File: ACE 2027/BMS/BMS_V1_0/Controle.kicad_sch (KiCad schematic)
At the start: 9 parts, among them J205 RJ45, J206 RJ45

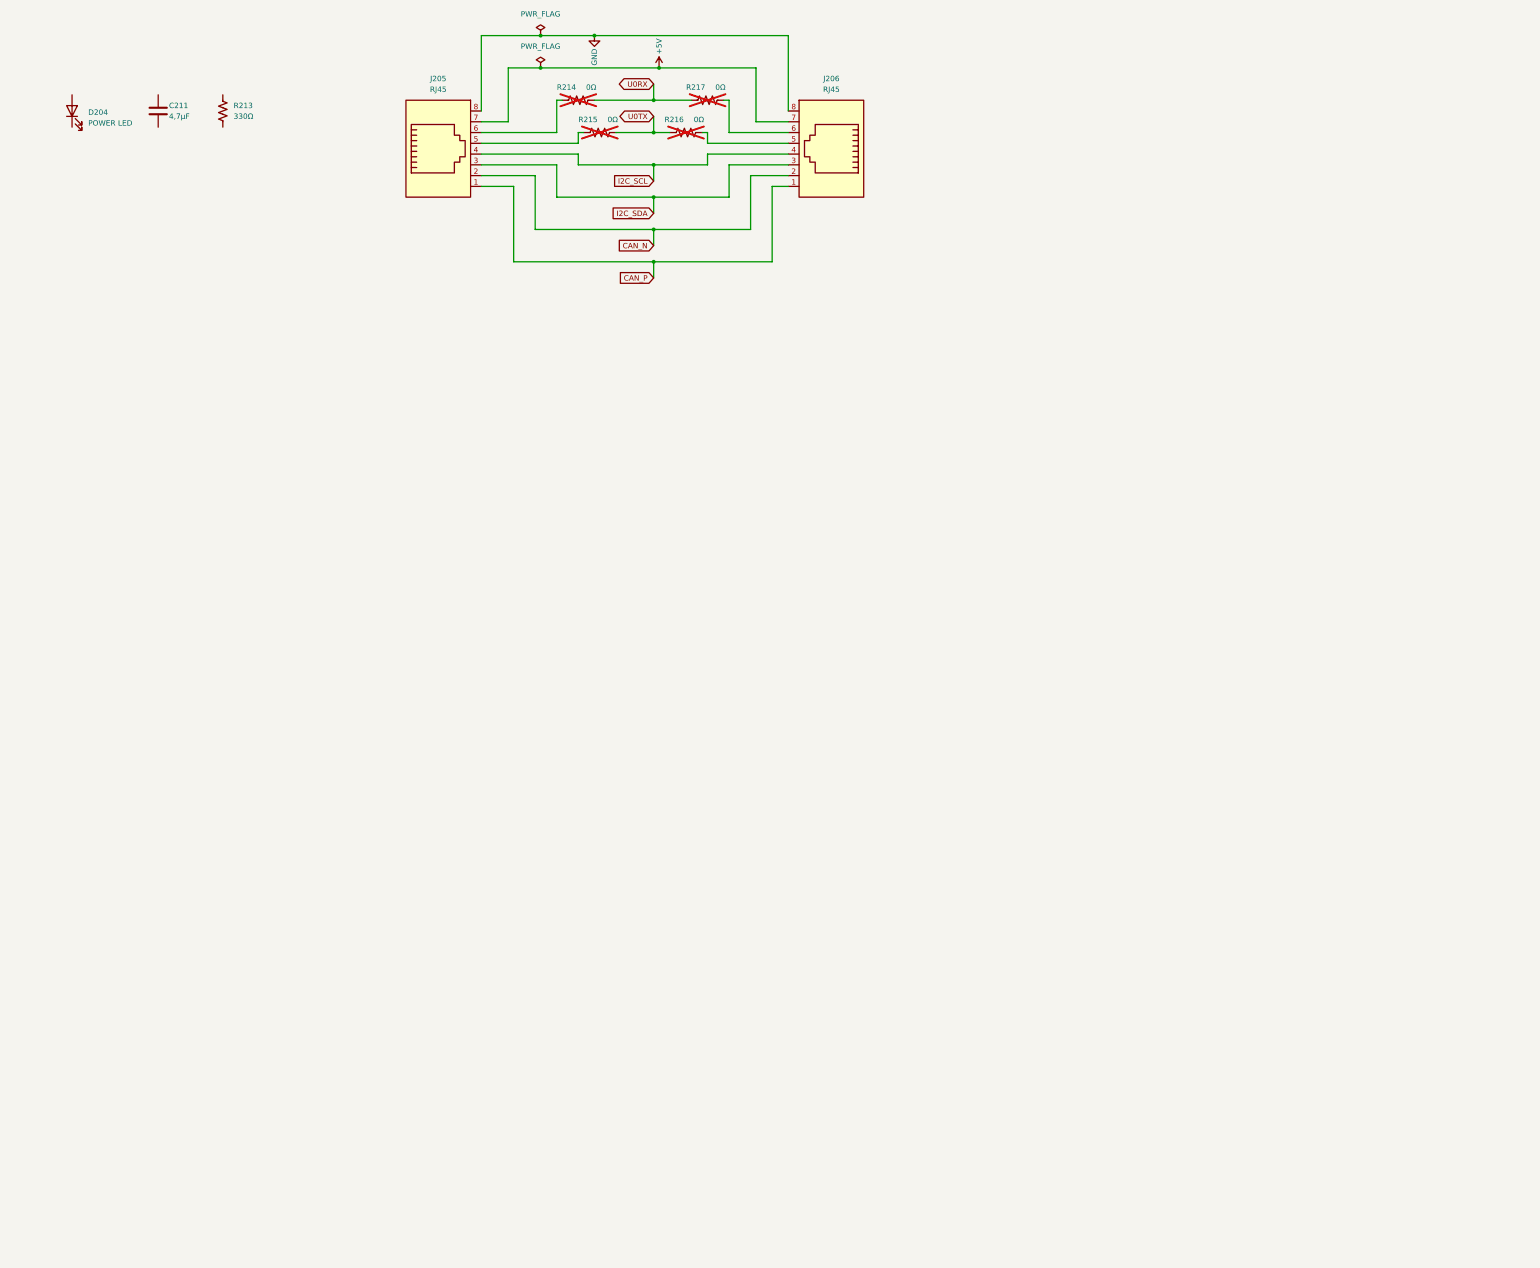
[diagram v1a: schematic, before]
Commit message: Avancement général du schémas
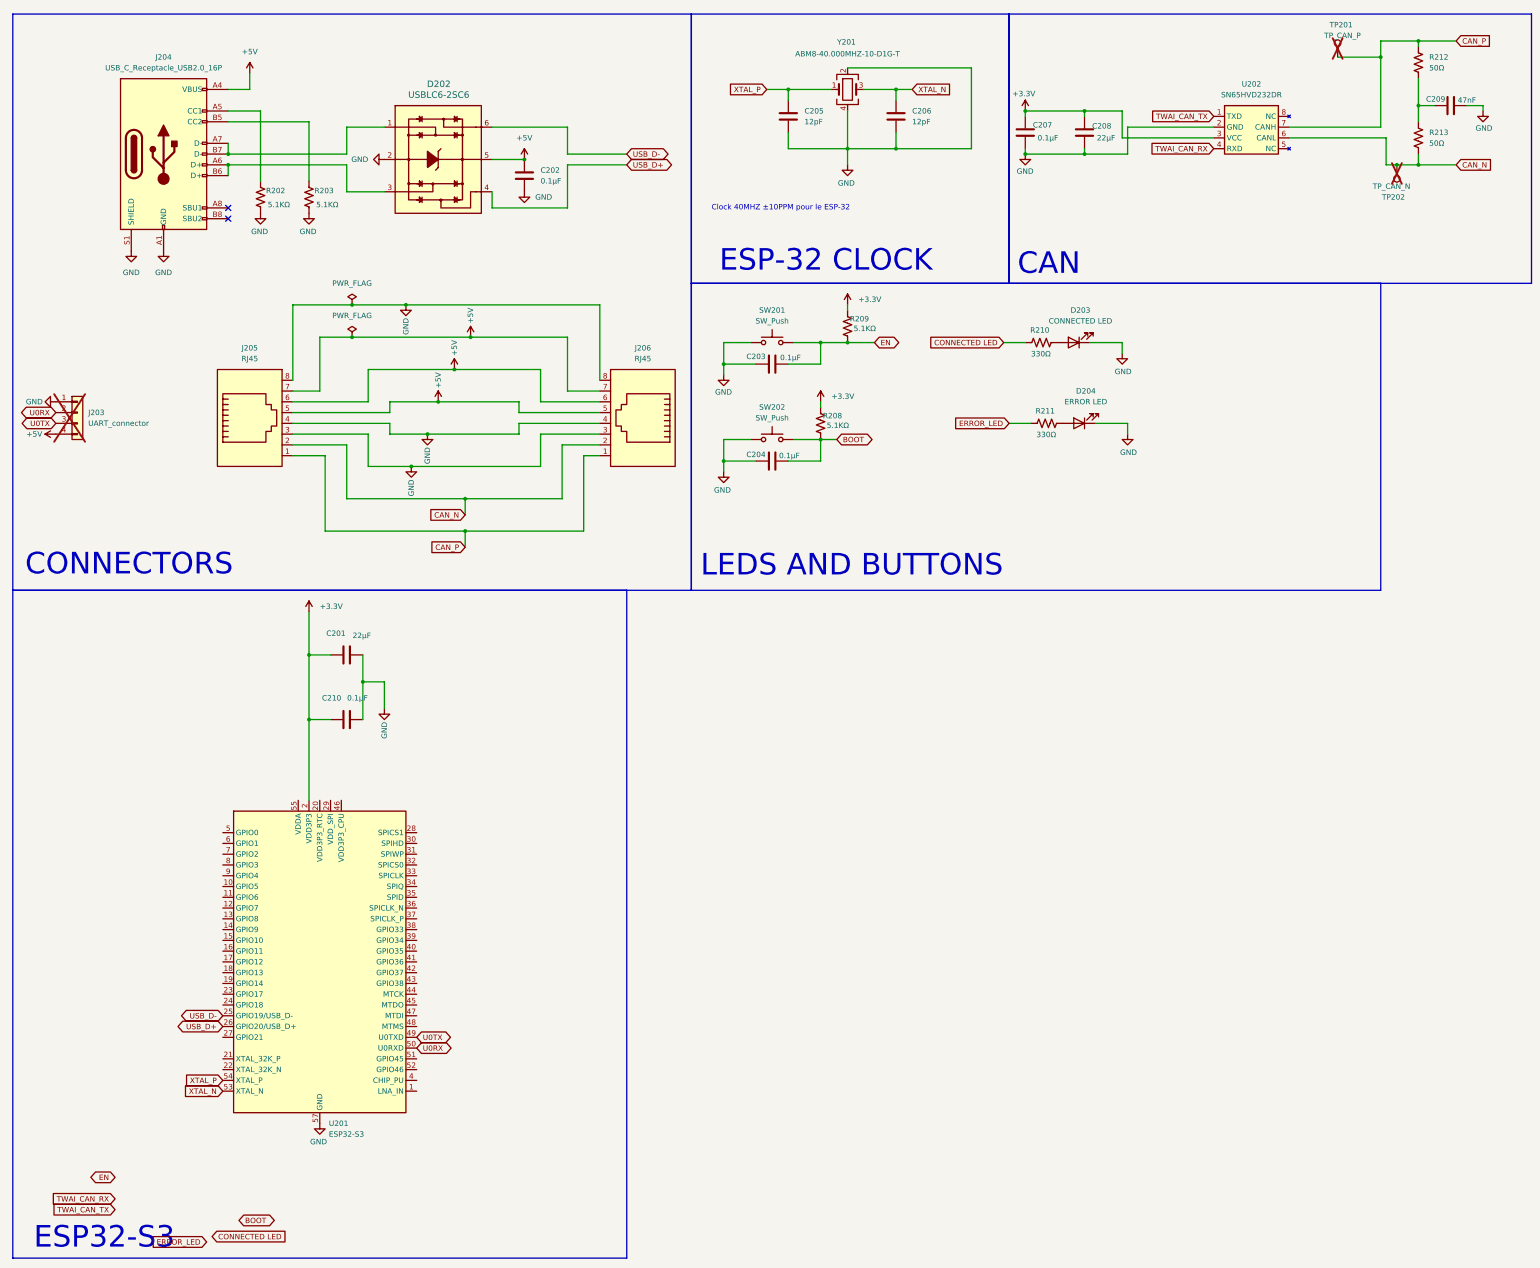
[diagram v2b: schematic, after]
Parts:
- removed C211: 4,7µF, Capacitor_SMD:C_0805_2012Metric_Pad1.18x1.45mm_HandSolder, symbol Device:C
- removed R214, R215, R216, R217: 0Ω, Resistor_SMD:R_0402_1005Metric_Pad0.72x0.64mm_HandSolder, symbol Device:R_US
- added C201, C208: 22μF, Capacitor_SMD:C_0805_2012Metric_Pad1.18x1.45mm_HandSolder, symbol Device:C
- added C202, C203, C204, C207, C210: 0.1μF, Capacitor_SMD:C_0805_2012Metric_Pad1.18x1.45mm_HandSolder, symbol Device:C
- added C205, C206: 12pF, Capacitor_SMD:C_0805_2012Metric_Pad1.18x1.45mm_HandSolder, symbol Device:C
- added C209: 47nF, Capacitor_SMD:C_0603_1608Metric_Pad1.08x0.95mm_HandSolder, symbol Device:C
- added D202: USBLC6-2SC6, BIMU:SOT23-6L, symbol BIMU_Custom:USBLC6-2SC6
- added D203: CONNECTED LED, LED_SMD:LED_0805_2012Metric_Pad1.15x1.40mm_HandSolder, symbol Device:LED
- added J203: UART_connector, Connector_PinSocket_2.54mm:PinSocket_1x04_P2.54mm_Vertical, symbol Connector_Generic:Conn_01x04
- added J204: USB_C_Receptacle_USB2.0_16P, Connector_USB:USB_C_Receptacle_GCT_USB4105-xx-A_16P_TopMnt_Horizontal, symbol Connector:USB_C_Receptacle_USB2.0_16P
- added R202, R203, R208, R209: 5.1KΩ, Resistor_SMD:R_0805_2012Metric_Pad1.20x1.40mm_HandSolder, symbol Device:R_US
- added R210, R211: 330Ω, Resistor_SMD:R_0805_2012Metric_Pad1.20x1.40mm_HandSolder, symbol Device:R_US
- added R212: 50Ω, Resistor_SMD:R_0805_2012Metric_Pad1.20x1.40mm_HandSolder, symbol Device:R_US
- added SW201, SW202: SW_Push, Button_Switch_SMD:SW_SPST_B3U-1000P, symbol Switch:SW_Push
- added TP201: TP_CAN_P, TestPoint:TestPoint_Pad_1.0x1.0mm, symbol Connector:TestPoint
- added TP202: TP_CAN_N, TestPoint:TestPoint_Pad_1.0x1.0mm, symbol Connector:TestPoint
- added U201: ESP32-S3, Package_DFN_QFN:QFN-56-1EP_7x7mm_P0.4mm_EP4x4mm, symbol MCU_Espressif:ESP32-S3
- added U202: SN65HVD232DR, Package_SO:SOIC-8_3.9x4.9mm_P1.27mm, symbol Motor_controller:SN65HVD232DR
- added Y201: ABM8-40.000MHZ-10-D1G-T, Crystal:Crystal_SMD_2016-4Pin_2.0x1.6mm, symbol Device:Crystal_GND24
- D204: value POWER LED -> ERROR LED; Digi-Key_PN 1516-QBLP631-IG5CT-ND -> 1516-QBLP631-R5-2897CT-ND
- R213: value 330Ω -> 50Ω; Digi-Key_PN 541-4168-1-ND -> 541-CRCW080550R0FKTACT-ND
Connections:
- net I2C_SCL is gone; now on net GND: J205.4, J206.4
- net I2C_SDA is gone; now on net GND: J205.3, J206.3
- net +5V: now also J205.5, J205.6, J206.5, J206.6, C202.1, D202.5, J203.4 (Pin_4), J204.A4 (VBUS), J204.A9 (VBUS), J204.B4 (VBUS), J204.B9 (VBUS)
- net CAN_N: now also R213.2, TP202.1, U202.6 (CANL)
- net CAN_P: now also R212.1, TP201.1, U202.7 (CANH)
- net GND: now also D204.1 (K), C201.2, C202.2, C203.2, C204.2, C205.2, C206.2, C207.2, C208.2, C209.1, C210.2, D202.2, D203.1 (K), J203.1 (Pin_1), J204.A1 (GND), J204.A12 (GND), J204.B1 (GND), J204.B12 (GND), J204.S1 (SHIELD), R202.2, R203.2, SW201.1, SW202.1, U201.57 (GND), U202.2 (GND), Y201.2, Y201.4
- net U0RX: now also J203.2 (Pin_2), U201.50 (U0RXD)
- net U0TX: now also J203.3 (Pin_3), U201.49 (U0TXD)
- net at D204.2 (A): now also R211.1
- net at R213.1: now also C209.2, R212.2
- new net: D203.2 (A), R210.1
- new net: J204.A5 (CC1), R202.1
- new net: J204.B5 (CC2), R203.1
- new net: U201.55 (VDDA), U201.56 (VDDA)
- new net: D202.3, J204.A6 (D+), J204.B6 (D+)
- new net: D202.1, J204.A7 (D-), J204.B7 (D-)
- new net +3.3V: C201.1, C207.1, C208.1, C210.1, R208.2, R209.2, U201.2 (VDD3P3), U201.3 (VDD3P3), U202.3 (VCC)
- new net BOOT: C204.1, R208.1, SW202.2
- new net CONNECTED LED: R210.2
- new net EN: C203.1, R209.1, SW201.2
- new net ERROR_LED: R211.2
- new net TWAI_CAN_RX: U202.4 (RXD)
- new net TWAI_CAN_TX: U202.1 (TXD)
- new net USB_D+: D202.4, U201.26 (GPIO20/USB_D+)
- new net USB_D-: D202.6, U201.25 (GPIO19/USB_D-)
- new net XTAL_N: C206.1, U201.53 (XTAL_N), Y201.3
- new net XTAL_P: C205.1, U201.54 (XTAL_P), Y201.1
- no-connect marks 0 -> 2
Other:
- note added: "CAN"
- note added: "CONNECTORS"
- note added: "Clock 40MHZ ±10PPM pour le ESP-32"
- note added: "ESP-32 CLOCK"
- note added: "ESP32-S3"
- note added: "LEDS AND BUTTONS"
